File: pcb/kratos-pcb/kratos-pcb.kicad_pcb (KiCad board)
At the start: 2 copper layers, 100 x 100 mm, 29 parts, among them IC2 SN74HC595N, J1 Barrel_Jack_Switch_Pin3Ring, Q2 2N2222A, Q3 2N2222A, SW1 SW_Push, U1 ESP32-DEVKIT-V1, U2 ULN2803A, U3 ULN2803A

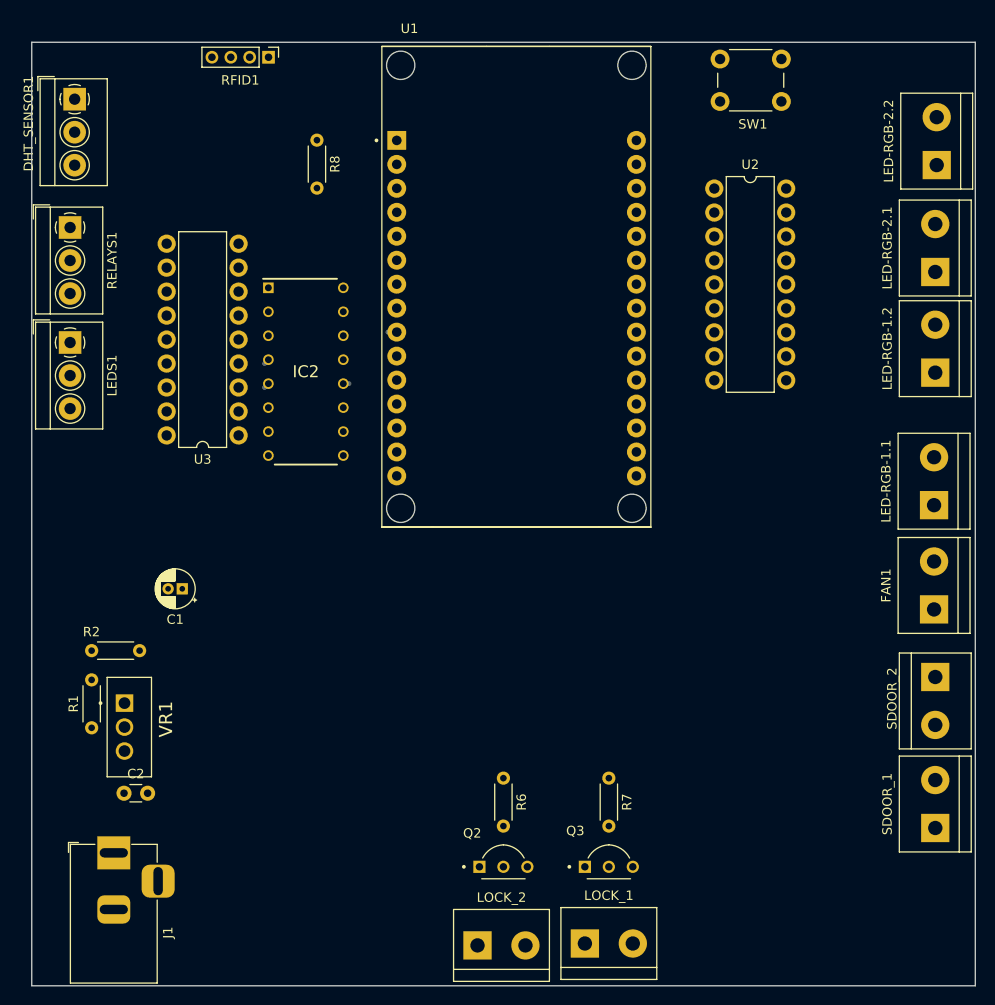
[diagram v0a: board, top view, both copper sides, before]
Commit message: ### modify
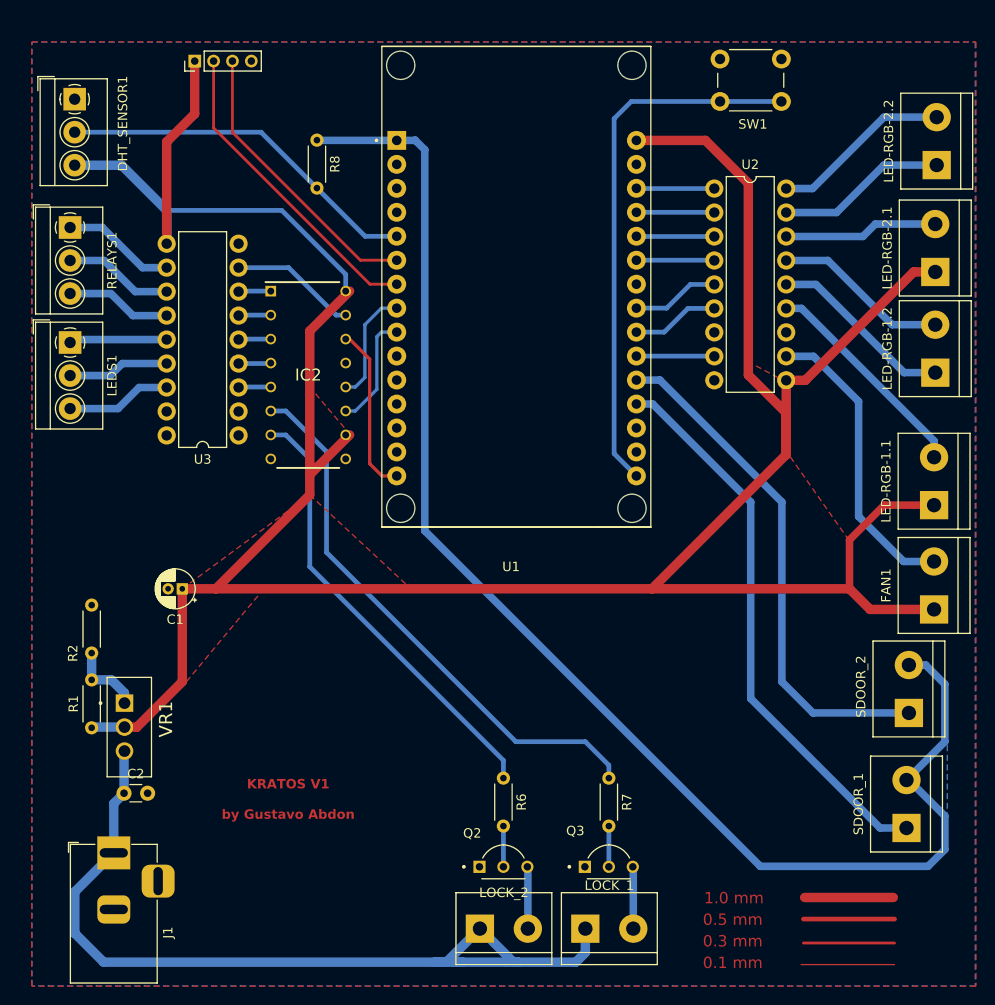
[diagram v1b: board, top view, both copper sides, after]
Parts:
- moved RFID1 7.83 mm to (111.3, 46.0), turned to 90 degrees
- moved R2 7.01 mm to (100.3, 103.6), turned to -90 degrees
- moved SDOOR_2 4.72 mm to (186.9, 115.1), turned to 90 degrees
- moved SDOOR_1 3.05 mm to (186.7, 127.3)
- moved LOCK_2 1.80 mm to (141.5, 137.9)
- moved LOCK_1 1.58 mm to (152.7, 137.9)
- moved IC2 0.44 mm to (123.3, 79.2)
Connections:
- IC2 pad 15: unconnected-(IC2-QA-Pad15) -> /EXPANSION DRIVERS/A
- RFID1 pad 2: RFID - TX -> RFID - RX
- RFID1 pad 3: RFID - RX -> RFID - TX
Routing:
- net +5V: track 0.81 -> 313.2 mm
- net +3.3V: track 0.04 -> 148.6 mm
- net +12V: track 0.15 -> 92.4 mm
- net SDOOR1: track 0.00 -> 59.4 mm
- net LOCKER_1: track 0.00 -> 59.0 mm
- net Net-(U1-EN): track 0.05 -> 57.4 mm
- net SDOOR2: track 0.00 -> 54.7 mm
- net LOCKER_2: track 0.00 -> 47.5 mm
- net DHT_DATA: track 0.00 -> 38.7 mm
- net (no net): track 0.00 -> 38.6 mm
- net RFID - RX: track 0.00 -> 33.4 mm
- net FAN_PWM: track 0.00 -> 31.8 mm
- net RFID - TX: track 0.00 -> 30.6 mm
- net Net-(LED-RGB-1.1-Pin_2): track 0.00 -> 23.2 mm
- net Net-(LED-RGB-1.2-Pin_1): track 0.00 -> 19.7 mm
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- added copper zone on B.Cu, net +12V
- added copper zone on B.Cu, net +3.3V
- added copper zone on F.Cu, net +5V
- added copper zone on B.Cu, net GND
- added copper zone on F.Cu, net GND
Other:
- board outline removed
- board text added: "0.1 mm"
- board text added: "0.3 mm"
- board text added: "0.5 mm"
- board text added: "1.0 mm"
- board text added: "KRATOS V1 by Gustavo Abdon"
